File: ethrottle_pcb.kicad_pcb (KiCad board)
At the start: 2 copper layers, 50 parts, among them J1 ATM15-08PA-BM02, K1 1462042-9, U1 LM4040DBZ-5, U2 LM324, U3 LM358_DFN, U4 LM324

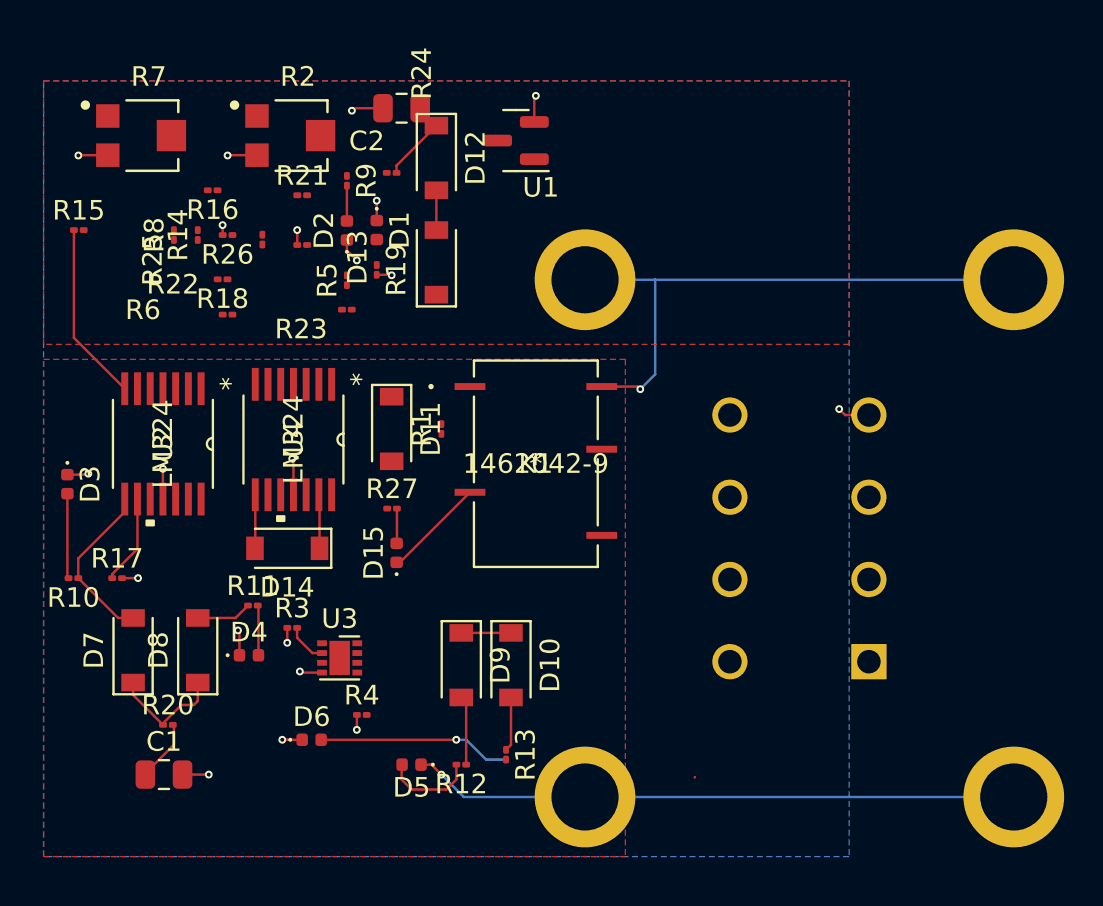
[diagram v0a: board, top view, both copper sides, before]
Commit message: update constraints
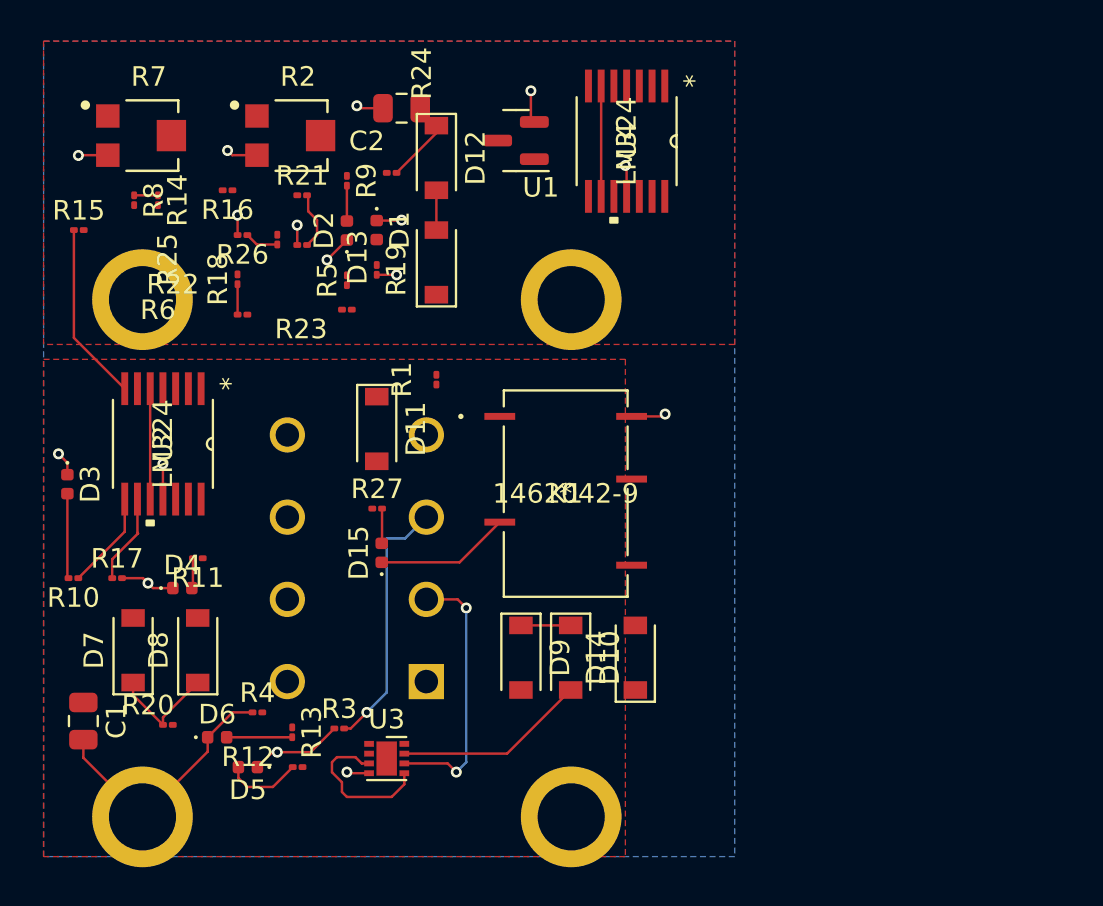
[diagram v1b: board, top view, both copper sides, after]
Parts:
- moved U4 22.8 mm to (128.8, 51.3)
- moved J1 22.6 mm to (118.6, 78.9)
- moved D14 18.6 mm to (129.3, 77.7), turned to 90 degrees
- moved R13 11.0 mm to (111.8, 81.5)
- moved D5 8.36 mm to (109.5, 83.3)
- moved R12 8.36 mm to (112.0, 83.3)
- moved R3 5.67 mm to (114.2, 81.3)
- moved U3 5.67 mm to (116.6, 82.9)
- moved R4 5.34 mm to (110.0, 80.5)
- moved C1 4.94 mm to (101.1, 81.0), turned to -90 degrees
- moved D4 4.83 mm to (106.1, 74.2)
- moved D6 4.83 mm to (107.9, 81.8)
- moved R11 3.71 mm to (106.9, 72.6), turned to 180 degrees
- moved D9 3.07 mm to (123.4, 77.7)
- moved D10 3.07 mm to (126.0, 77.7)
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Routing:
- net GND: track 84.4 -> 40.5 mm, vias 22 -> 16
- net Brake: track 2.10 -> 18.9 mm, vias 0 -> 1
- net Throttle: track 0.00 -> 13.7 mm, vias 0 -> 2
- net 0.5V: track 0.00 -> 11.0 mm
- net Net-(R25-Pad2): track 0.00 -> 7.37 mm
- net Net-(D10-Pad2): track 2.78 -> 9.84 mm
- net Net-(D6-Pad2): track 9.86 -> 3.35 mm, vias 1 -> 0
- net Net-(D7-Pad2): track 9.42 -> 5.02 mm
- net Net-(D9-Pad2): track 3.53 -> 0.00 mm
- net Net-(C1-Pad1): track 5.71 -> 2.54 mm
- net Net-(D8-Pad2): track 2.83 -> 0.00 mm
- net Net-(D13-Pad1): track 2.75 -> 0.00 mm
- net Net-(D14-Pad2): track 2.74 -> 0.00 mm
- net Net-(D15-Pad1): track 5.23 -> 6.88 mm
- net +5V: track 0.00 -> 1.56 mm
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
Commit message: more traces
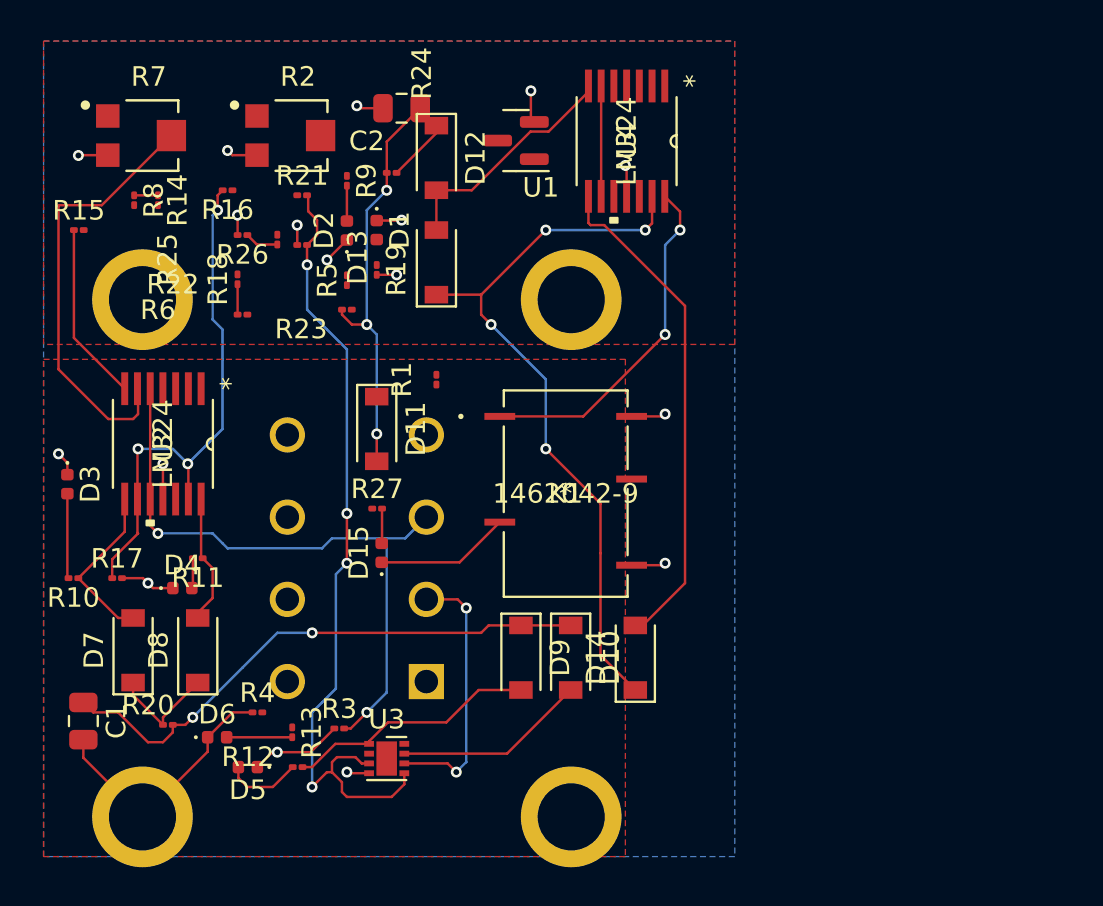
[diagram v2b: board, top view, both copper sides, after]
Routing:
- net Net-(D13-Pad1): track 0.00 -> 37.4 mm, vias 0 -> 4
- net 0.5V: track 11.0 -> 41.5 mm, vias 0 -> 4
- net Net-(C1-Pad1): track 2.54 -> 28.4 mm, vias 0 -> 2
- net Net-(D14-Pad2): track 0.00 -> 25.6 mm
- net 4.5V: track 4.60 -> 27.0 mm, vias 0 -> 3
- net BREF: track 0.00 -> 22.2 mm
- net Net-(C2-Pad1): track 0.00 -> 21.1 mm, vias 0 -> 3
- net Net-(K1-Pad1): track 0.00 -> 17.9 mm, vias 0 -> 2
- net Brake: track 18.9 -> 33.0 mm, vias 1 -> 2
- net Net-(D9-Pad2): track 0.00 -> 12.9 mm
- net Net-(D12-Pad2): track 2.03 -> 12.2 mm
- net Net-(D8-Pad2): track 0.00 -> 6.63 mm
- net Net-(D7-Pad2): track 5.02 -> 8.66 mm
- net GND: track 40.5 -> 42.3 mm, vias 16 -> 17
